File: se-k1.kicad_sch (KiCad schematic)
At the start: 38 parts, among them J1 USB_C_Receptacle_USB2.0_14P, U1 ESP32-S3-MINI-1U, U3 W25Q16JVSSIQ, U4 AMS1117-3.3

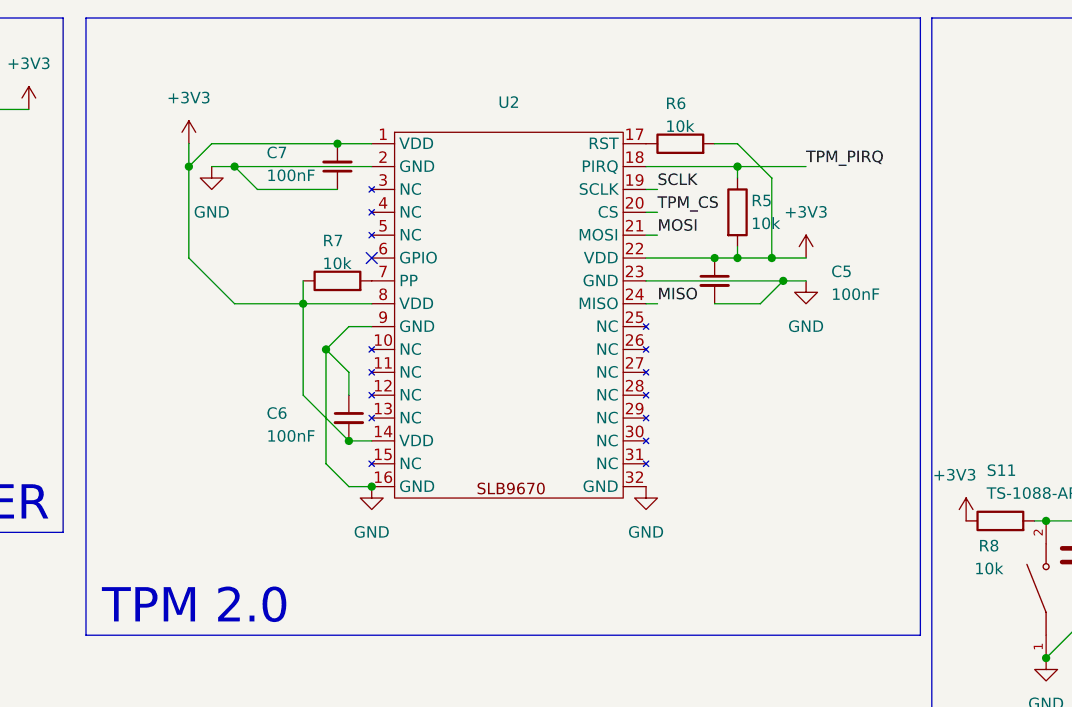
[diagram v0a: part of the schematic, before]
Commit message: finish!
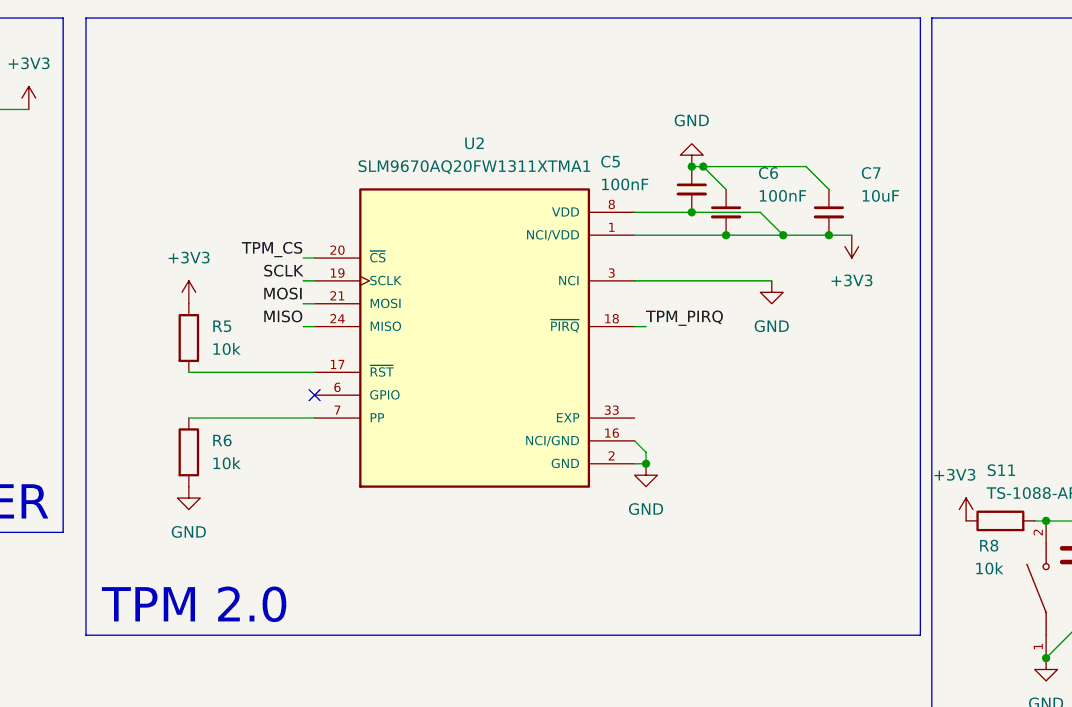
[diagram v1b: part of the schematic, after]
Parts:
- removed R7: 10k, Resistor_SMD:R_0402_1005Metric, symbol Device:R
- removed U2: ~, SLB9670VQ20FW785XUMA1:QFN50P500X500X90-33N, symbol tpm:SLB9670
- added U2: SLM9670AQ20FW1311XTMA1, SLM9670AQ20FW1311XTMA1:QFN50P500X500X90-33N, symbol SLM9670AQ20FW1311XTMA1:SLM9670AQ20FW1311XTMA1
- C1, C3, C4, C5, C6: footprint Capacitor_SMD:C_0805_2012Metric -> Capacitor_SMD:C_0402_1005Metric
- C7: value 100nF -> 10uF; footprint Capacitor_SMD:C_0805_2012Metric -> Capacitor_SMD:C_0402_1005Metric
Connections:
- net +3V3: now also C5.2, R5.1, U2.1 (NCI/VDD), U2.14 (NCI/VDD), U2.22 (VDD), U2.8 (VDD); no longer C5.1, R5.2, R6.2
- net GND: now also C5.1, R6.2, U2.10 (NCI), U2.11 (NCI), U2.12 (NCI), U2.13 (NCI), U2.15 (NCI), U2.16 (NCI/GND), U2.2 (GND), U2.23 (GND), U2.25 (NCI), U2.26 (NCI), U2.27 (NCI), U2.28 (NCI), U2.3 (NCI), U2.31 (NCI), U2.32 (GND), U2.4 (NCI), U2.5 (NCI), U2.9 (GND); no longer C5.2
- net MISO: now also U2.24 (MISO)
- net MOSI: now also U2.21 (MOSI)
- net SCLK: now also U2.19 (SCLK)
- net TPM_CS: now also U2.20 (~{CS})
- net TPM_PIRQ: now also U2.18 (~{PIRQ}); no longer R5.1
- net at R6.1: now also U2.7 (PP)
- new net: R5.2, U2.17 (~{RST})
